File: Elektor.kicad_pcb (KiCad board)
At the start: 2 copper layers, 50 x 44 mm, 55 parts, among them J1 Conn_Coaxial, J13 Conn_Coaxial, J6 Conn_01x03_Pin, J8 Conn_01x02, Q1 BF545B, U1 Si5351A-B-GT, U2 74HC04, U3 74HC4066D_653, U5 MCP6022, U6 AUDIOSHIELD-REVD, U7 MCP6022, Y1 ABM7-25.000MHZ-D2Y-T

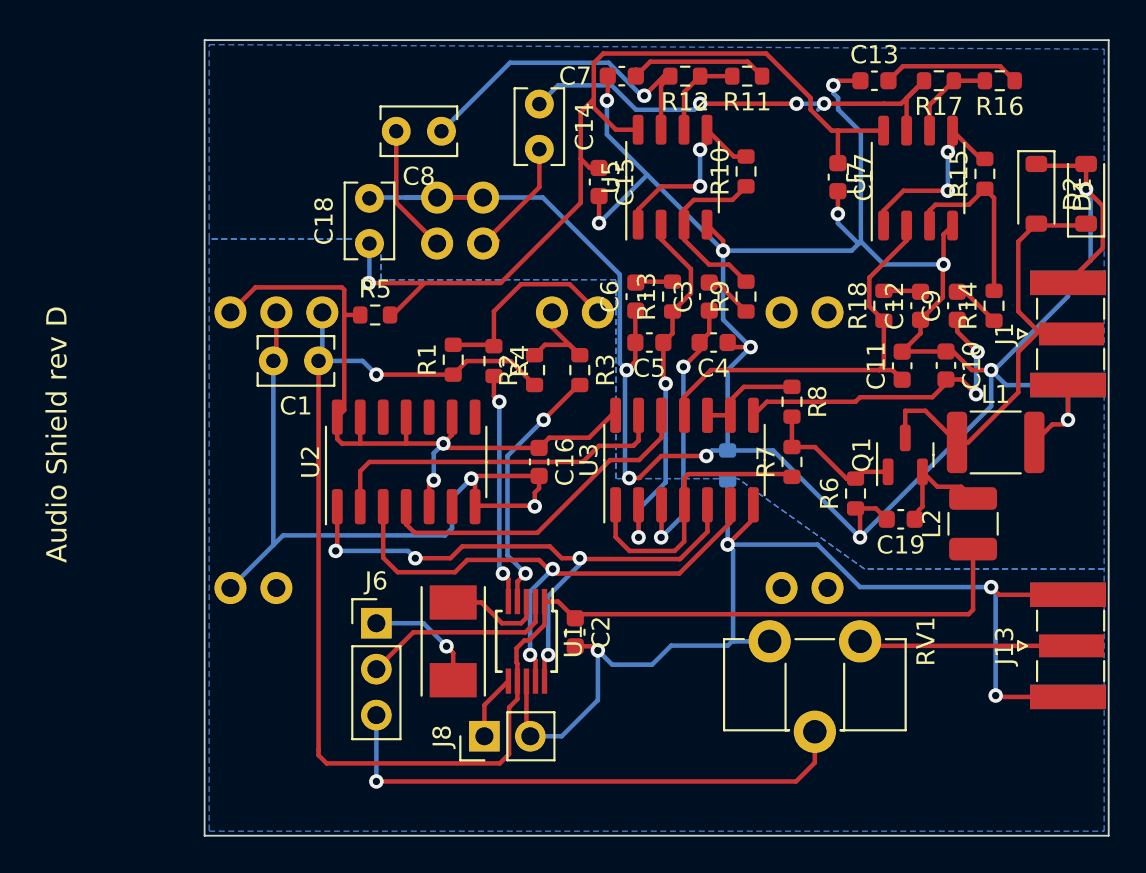
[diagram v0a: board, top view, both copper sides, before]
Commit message: alternative layout first commit
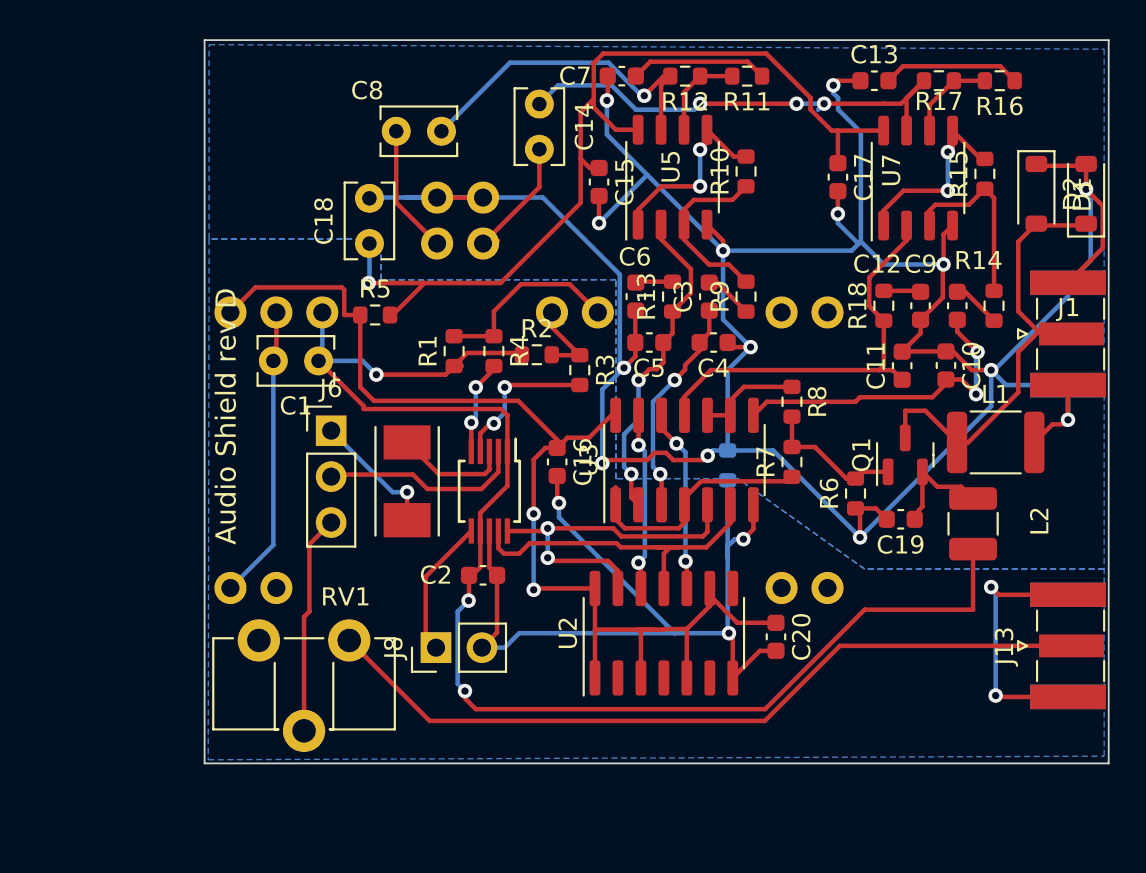
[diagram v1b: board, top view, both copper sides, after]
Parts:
- added C20: 100n, Capacitor_SMD:C_0603_1608Metric, F.Cu at (188.6, 94.0)
- moved RV1 28.3 mm to (165.0, 94.2)
- moved U2 17.1 mm to (182.4, 93.8)
- moved J6 10.9 mm to (164.0, 82.6)
- moved Y1 9.21 mm to (168.2, 85.4)
- moved U1 8.55 mm to (172.8, 86.0)
- moved C2 5.99 mm to (172.4, 90.6), turned to 0 degrees
- moved J8 5.58 mm to (169.8, 94.6)
- moved C16 1.00 mm to (176.5, 84.3)
- moved R2 0.86 mm to (175.4, 78.4), turned to 0 degrees
- moved R4 0.55 mm to (173.0, 78.2)
- moved R1 0.48 mm to (170.8, 78.2)
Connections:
- U2 pad 1: Net-(U1-CLK0) -> Net-(U2G-VCC)
- U2 pad 10: unconnected-(U2-Pad10) -> Net-(U3-4E)
- U2 pad 11: Net-(U2G-VCC) -> Net-(U1-CLK1)
- U2 pad 12: unconnected-(U2-Pad12) -> Net-(U3-1E)
- U2 pad 13: Net-(U2G-VCC) -> Net-(U1-CLK0)
- U2 pad 2: Net-(U3-1E) -> unconnected-(U2-Pad2)
- U2 pad 3: Net-(U1-CLK1) -> Net-(U2G-VCC)
- U2 pad 4: Net-(U3-4E) -> unconnected-(U2-Pad4)
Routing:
- net Net-(J13-In): track 12.9 -> 44.6 mm
- net Net-(U2G-VCC): track 41.0 -> 65.6 mm
- net GND: track 106.5 -> 83.4 mm, vias 6 -> 5
- net Net-(J6-Pin_3): track 30.1 -> 12.1 mm, vias 1 -> 0
- net Net-(U1-CLK0): track 33.6 -> 19.7 mm, vias 4 -> 2
- net Net-(U1-CLK1): track 31.9 -> 19.1 mm, vias 2 -> 0
- net Net-(U3-1E): track 19.5 -> 10.1 mm, vias 0 -> 2
- net Net-(U3-4E): track 18.7 -> 10.2 mm, vias 0 -> 2
- net 3.3V: track 86.1 -> 78.5 mm, vias 1 -> 3
- net Net-(U1-SDA): track 12.8 -> 5.24 mm
- net Net-(U1-SCL): track 14.3 -> 8.43 mm
- net Net-(J8-Pin_1): track 3.60 -> 7.73 mm
- net Net-(U3-2Z): track 16.3 -> 12.2 mm
- net Net-(U3-1Z): track 21.1 -> 18.3 mm
- net Net-(U3-1Y): track 15.7 -> 13.7 mm
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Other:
- board size 50 x 44 mm -> 50 x 40 mm
